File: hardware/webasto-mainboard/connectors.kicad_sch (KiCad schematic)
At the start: 5 parts

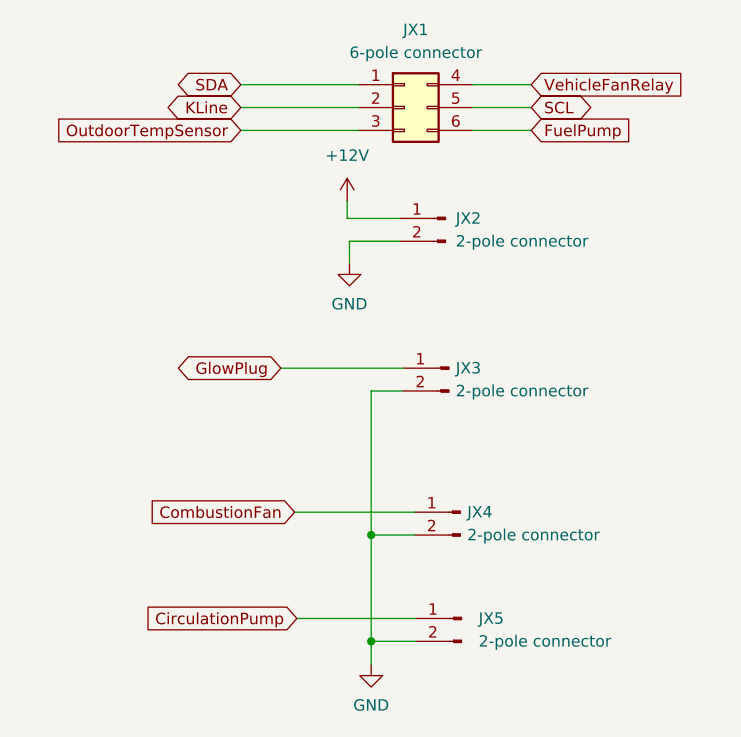
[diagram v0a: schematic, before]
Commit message: v1.0 layout complete
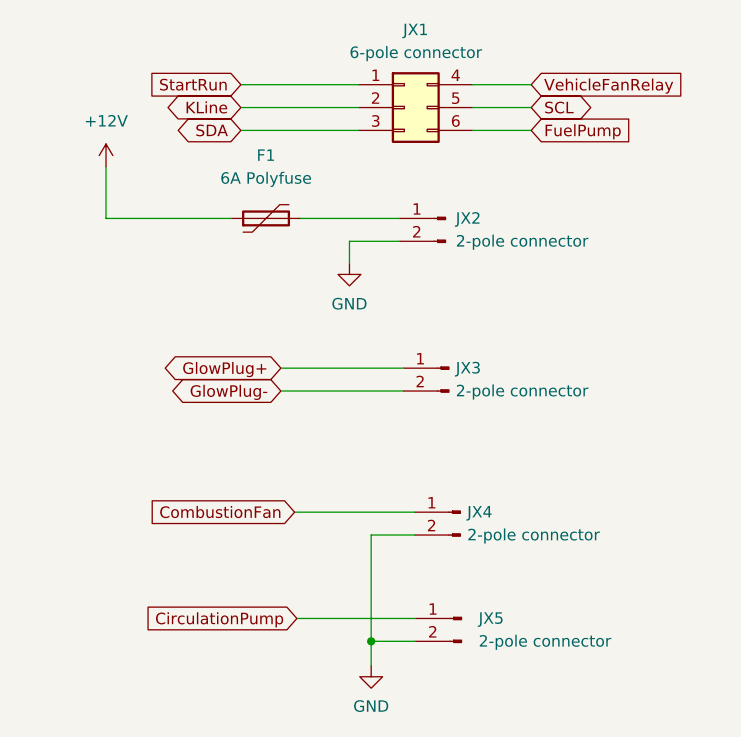
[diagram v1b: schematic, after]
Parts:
- added F1: 6A Polyfuse, Resistor_SMD:R_0603_1608Metric_Pad0.98x0.95mm_HandSolder, symbol Device:Polyfuse
- JX1: footprint (none) -> Beirdo:Webasto_Therma_Top_C_X1
- JX2: footprint (none) -> Beirdo:Webasto_Therma_Top_C_X2
- JX3: footprint (none) -> Beirdo:Webasto_Therma_Top_C_X3
- JX4, JX5: footprint (none) -> Beirdo:Webasto_Therma_Top_C_X4X5
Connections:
- net OutdoorTempSensor is gone; now on net SDA: JX1.3 (Pin_3)
- net +12V: now also F1.1; no longer JX2.1 (Pin_1)
- net GND: no longer JX3.2 (Pin_2)
- net SDA: no longer JX1.1 (Pin_1)
- net GlowPlug renamed GlowPlug+
- new net: F1.2, JX2.1 (Pin_1)
- new net GlowPlug-: JX3.2 (Pin_2)
- new net StartRun: JX1.1 (Pin_1)
